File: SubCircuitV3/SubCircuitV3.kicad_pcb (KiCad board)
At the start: 2 copper layers, 120 x 120.1 mm, 26 parts, among them J1 JTAG, J10 ESC_POWER, J11 ESC_POWER, J12 ESC_POWER, J13 ESC_POWER, J14 FEMALE XT-60, J15 ESC PWM, J16 3S, J2 ESC PWM, J3 ESC PWM, J4 ESC PWM, J5 ESC PWM, J6 ESC PWM, J7 5S, J8 ESC_POWER, J9 ESC_POWER, K1 G5Q-1A

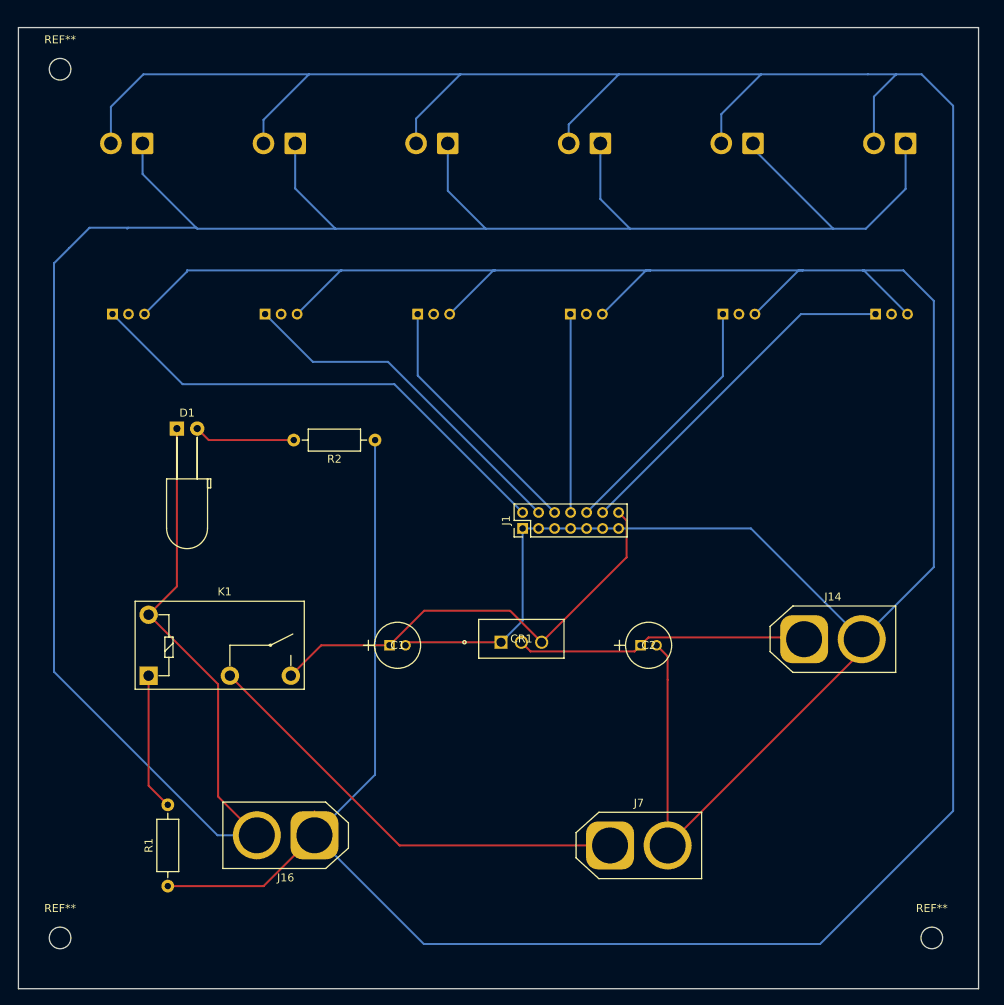
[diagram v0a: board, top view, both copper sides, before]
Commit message: Finalized V3 Board
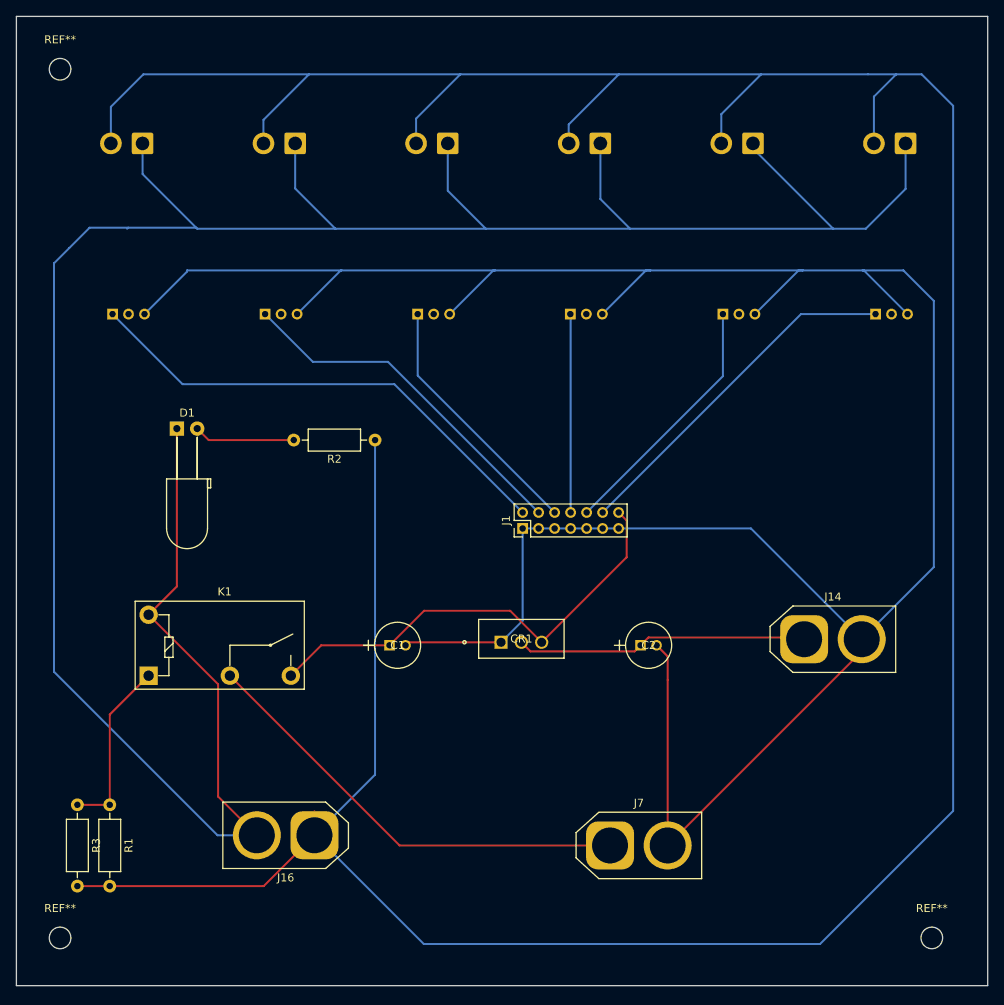
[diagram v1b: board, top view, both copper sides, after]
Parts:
- added R3: 1000, Resistor_THT:R_Axial_DIN0207_L6.3mm_D2.5mm_P10.16mm_Horizontal, F.Cu at (107.3, 124.1)
- R1: value 2000 -> 1000
- moved R1 12.5 mm to (111.4, 124.1), turned to -90 degrees
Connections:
- J1 pad 14: Net-(CR1-INPUT) -> Net-(CR1-OUTPUT)
- R1 pad 1: +12V -> Net-(K1-Pad1)
- R1 pad 2: Net-(K1-Pad1) -> +12V
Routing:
- net +12V: track 424.2 -> 435.5 mm
- net Net-(K1-Pad1): track 17.1 -> 22.2 mm
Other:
- board size 120 x 120.1 mm -> 121.4 x 121.2 mm
